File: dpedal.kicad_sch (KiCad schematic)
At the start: 3 parts

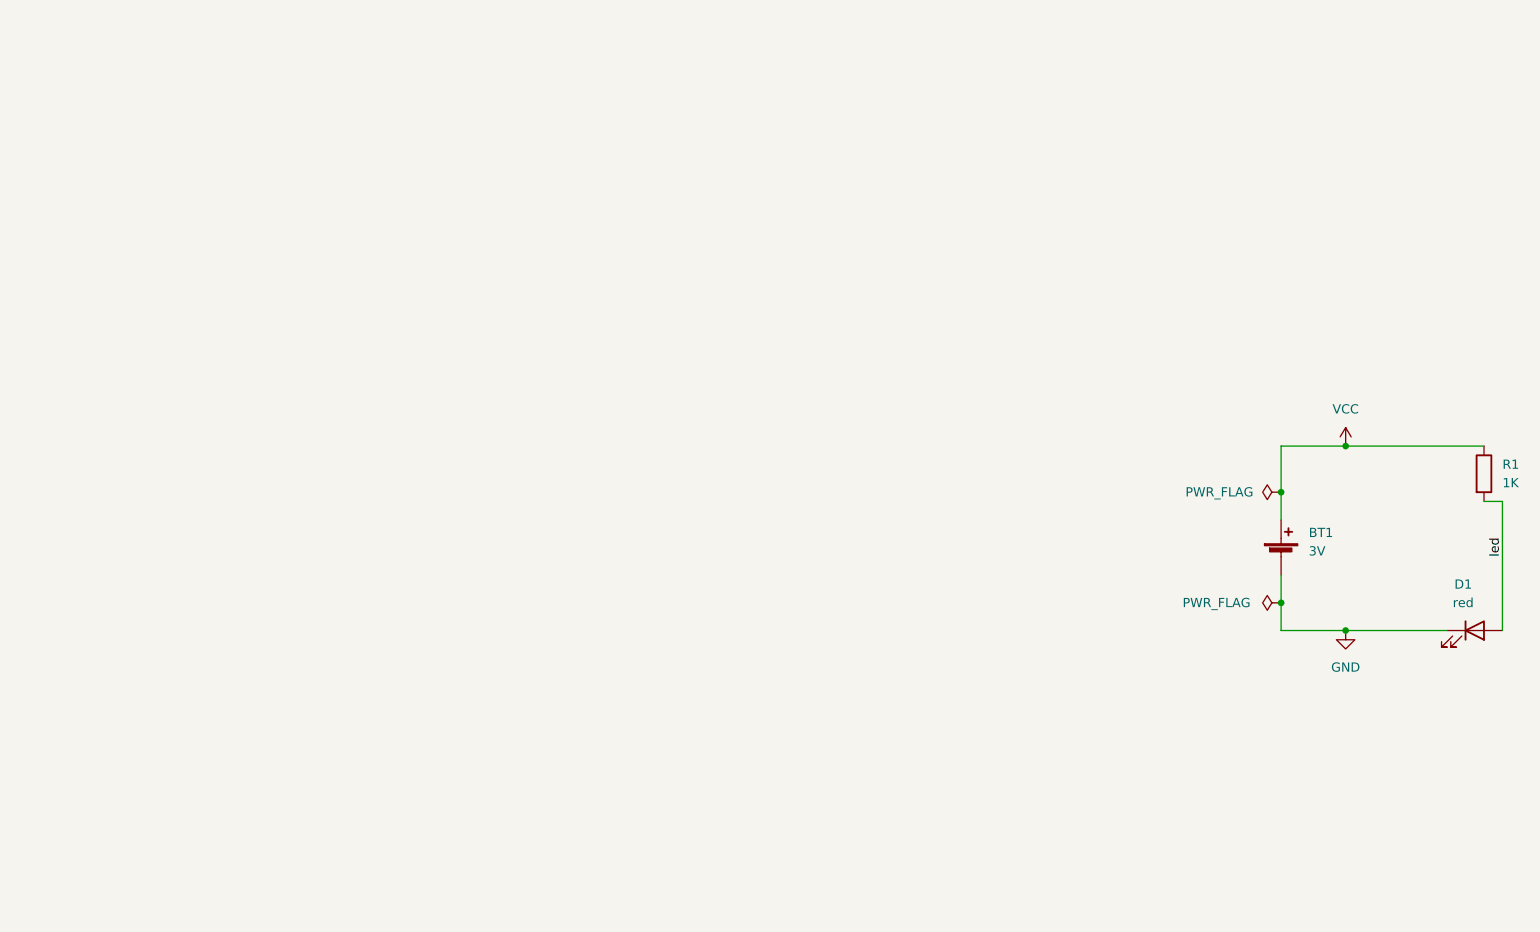
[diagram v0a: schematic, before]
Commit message: progress
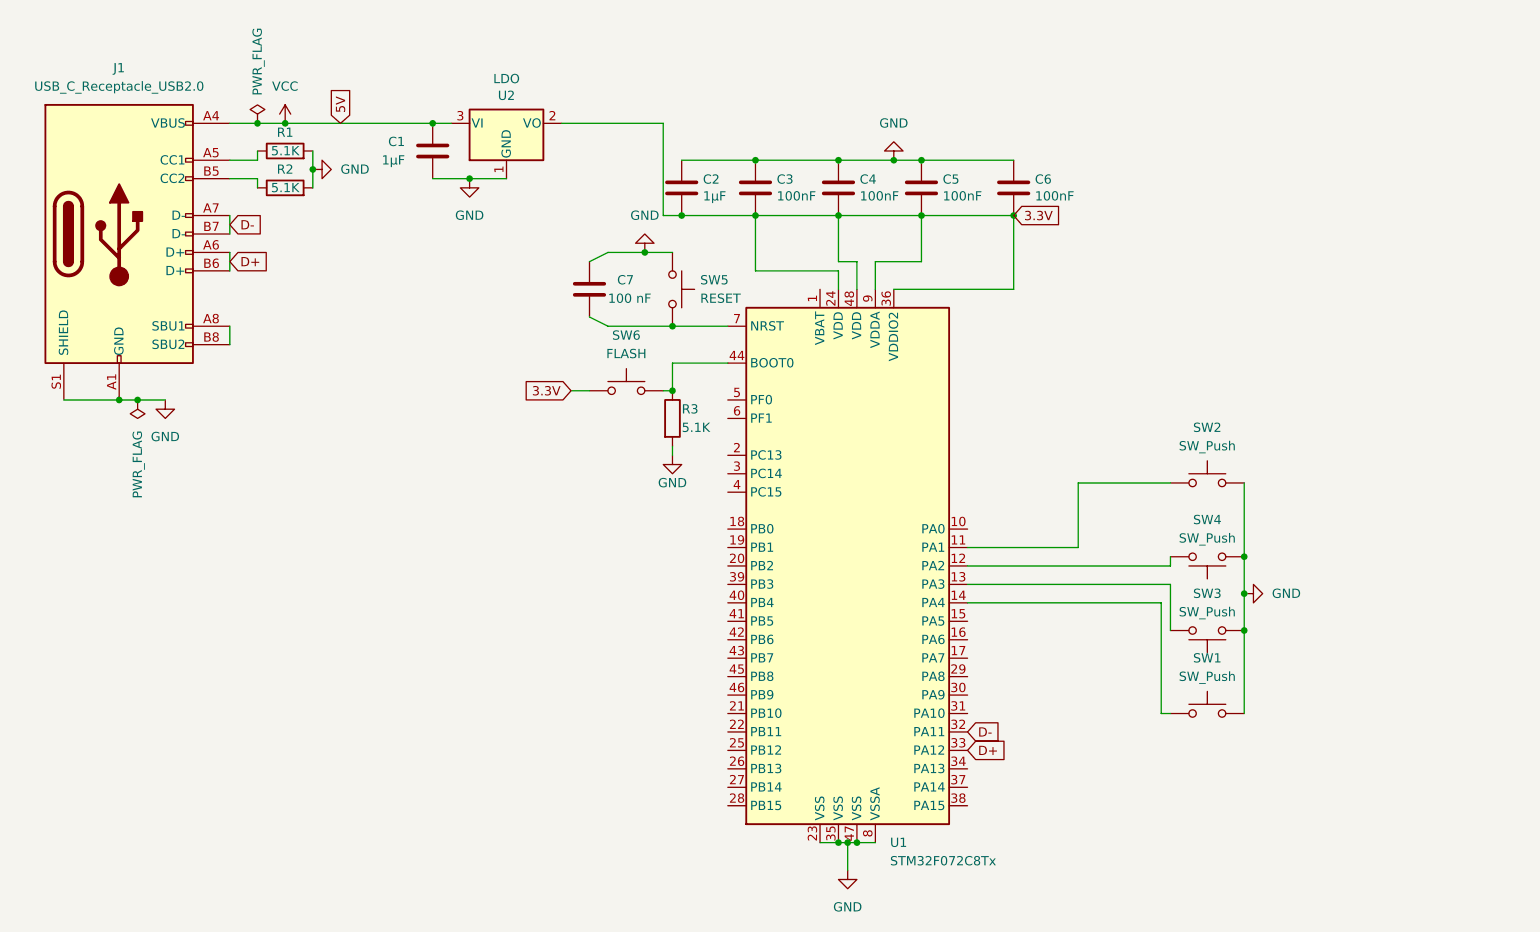
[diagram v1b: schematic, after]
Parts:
- removed BT1: 3V, Battery:BatteryHolder_Keystone_1058_1x2032, symbol Device:Battery_Cell
- removed D1: red, LED_THT:LED_D5.0mm, symbol Device:LED
- added C1, C2: 1µF, Capacitor_SMD:C_0402_1005Metric, symbol Device:C
- added C3, C4, C5, C6: 100nF, Capacitor_SMD:C_0402_1005Metric, symbol Device:C
- added C7: 100 nF, Capacitor_SMD:C_0402_1005Metric, symbol Device:C
- added J1: USB_C_Receptacle_USB2.0, Connector_USB:USB_C_Receptacle_HRO_TYPE-C-31-M-12, symbol Connector:USB_C_Receptacle_USB2.0
- added R2, R3: 5.1K, Resistor_SMD:R_0402_1005Metric, symbol Device:R
- added SW1, SW2, SW3, SW4: SW_Push, Button_Switch_Keyboard:SW_Cherry_MX_1.00u_Plate, symbol Switch:SW_Push
- added SW5: RESET, Button_Switch_SMD:SW_SPST_CK_RS282G05A3, symbol Switch:SW_Push
- added SW6: FLASH, Button_Switch_SMD:SW_SPST_CK_RS282G05A3, symbol Switch:SW_Push
- added U1: STM32F072C8Tx, Package_QFP:LQFP-48_7x7mm_P0.5mm, symbol MCU_ST_STM32F0:STM32F072C8Tx
- added U2: LDO, Package_TO_SOT_SMD:SOT-23, symbol Regulator_Linear:MCP1703A-3302_SOT23
- R1: value 1K -> 5.1K; footprint Resistor_THT:R_Axial_DIN0309_L9.0mm_D3.2mm_P12.70mm_Horizontal -> Resistor_SMD:R_0402_1005Metric
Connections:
- net led is gone; now on net GND: R1.2
- net GND: now also C1.1, C2.1, C3.1, C4.1, C5.1, C6.1, C7.1, J1.A1 (GND), J1.A12 (GND), J1.B1 (GND), J1.B12 (GND), J1.S1 (SHIELD), R2.2, R3.2, SW1.2, SW2.2, SW3.1, SW4.1, SW5.1, U1.23 (VSS), U1.35 (VSS), U1.47 (VSS), U1.8 (VSSA), U2.1 (GND)
- net VCC: now also C1.2, J1.A4 (VBUS), J1.A9 (VBUS), J1.B4 (VBUS), J1.B9 (VBUS), U2.3 (VI); no longer R1.1
- new net: J1.A5 (CC1), R1.1
- new net: J1.A8 (SBU1), J1.B8 (SBU2)
- new net: J1.B5 (CC2), R2.1
- new net: SW4.2, U1.12 (PA2)
- new net: R3.1, SW6.2, U1.44 (BOOT0)
- new net: SW2.1, U1.11 (PA1)
- new net: SW3.2, U1.13 (PA3)
- new net: SW1.1, U1.14 (PA4)
- new net: C7.2, SW5.2, U1.7 (NRST)
- new net 3.3V: C2.2, C3.2, C4.2, C5.2, C6.2, SW6.1, U1.24 (VDD), U1.36 (VDDIO2), U1.48 (VDD), U1.9 (VDDA), U2.2 (VO)
- new net D+: J1.A6 (D+), J1.B6 (D+), U1.33 (PA12)
- new net D-: J1.A7 (D-), J1.B7 (D-), U1.32 (PA11)
